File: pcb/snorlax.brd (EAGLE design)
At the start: 36.5 x 29.2 mm, 13 parts, among them IC1 MCP3008

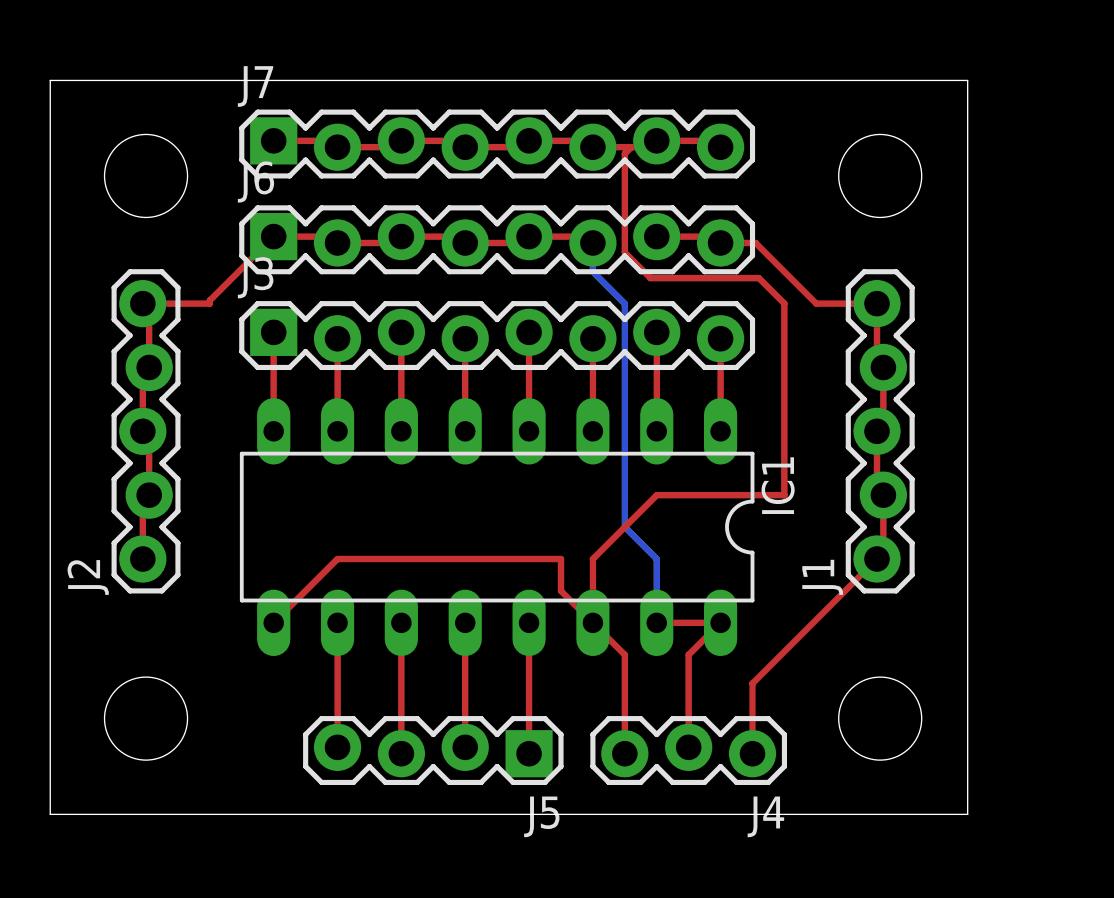
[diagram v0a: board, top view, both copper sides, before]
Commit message: Final PCB Schematics, Board Layouts and Gerber Files
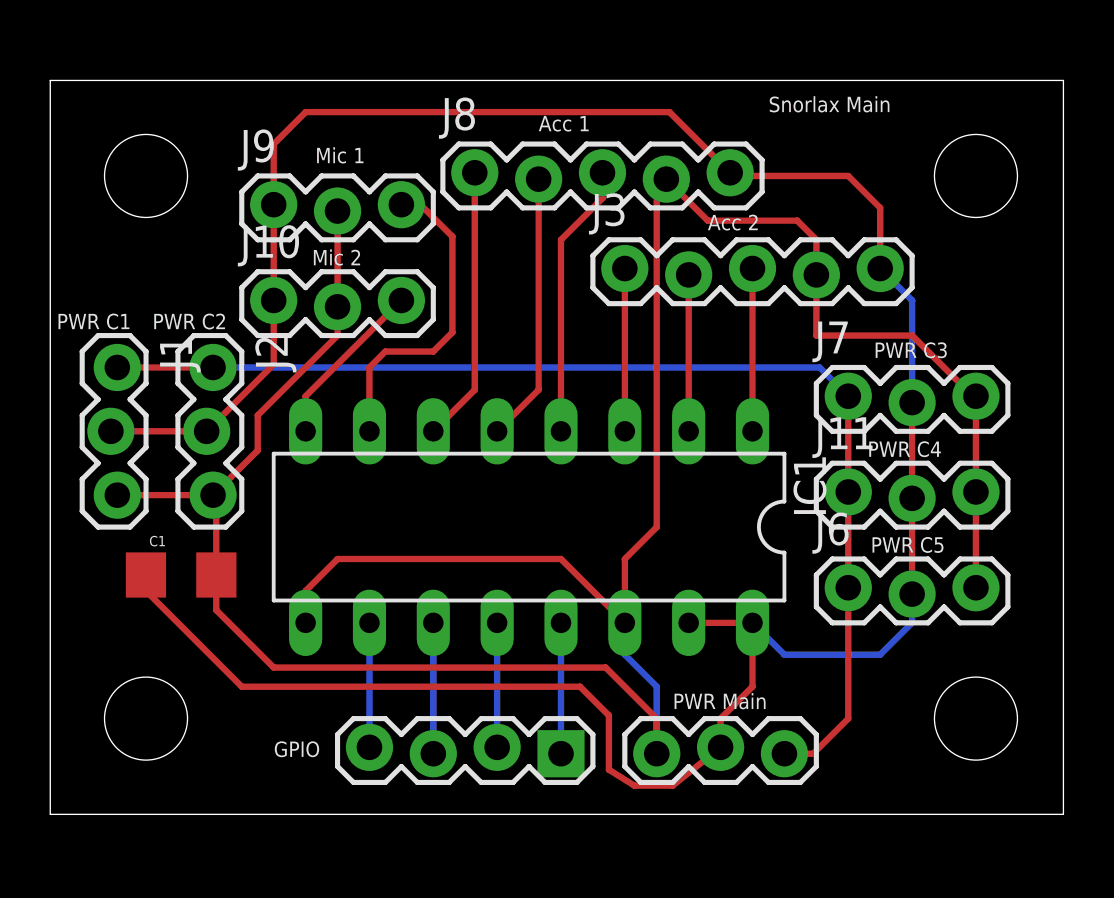
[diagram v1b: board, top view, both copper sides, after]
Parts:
- added C1: 22uF, SparkFun-Capacitors:1206
- added J10, J11, J9: (no value), SparkFun-Connectors:1X03_LOCK
- added J8: (no value), SparkFun-Connectors:1X05_LOCK
- J1, J2: device SparkFun-Connectors:1X05_LOCK -> SparkFun-Connectors:1X03_LOCK
- J3: device SparkFun-Connectors:1X08_LOCK -> SparkFun-Connectors:1X05_LOCK
- J6, J7: device SparkFun-Connectors:1X08_LOCK -> SparkFun-Connectors:1X03_LOCK
- moved J1 31.4 mm to (2.54, 17.8), turned to 270 degrees
- moved J6 26.8 mm to (31.8, 8.89)
- moved J7 25.0 mm to (31.8, 16.5)
- moved J3 14.2 mm to (22.9, 21.6)
- moved J2 8.03 mm to (6.35, 17.8), turned to 270 degrees
- moved H3 3.81 mm to (36.8, 25.4)
- moved H4 3.81 mm to (36.8, 3.81)
- moved IC1 1.27 mm to (19.1, 11.4)
- moved J4 1.27 mm to (29.2, 2.54)
- moved J5 1.27 mm to (20.3, 2.54)
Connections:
- net GND: now also C1.2, J1.3, J10.2, J11.3, J2.3, J3.4, J6.3, J8.4, J9.2; no longer J7.1, J7.2, J7.4, J7.5, J7.6, J7.7, J7.8
- net N$1: now also J3.3; no longer J3.8
- net N$2: now also J3.2; no longer J3.7
- net N$3: now also J3.1; no longer J3.6
- net N$4: now also J8.3; no longer J3.5
- net N$5: now also J8.2; no longer J3.4
- net N$6: now also J8.1; no longer J3.3
- net N$7: now also J9.3; no longer J3.2
- net N$8: now also J10.3; no longer J3.1
- net VCC_3.3: now also C1.1, J1.2, J10.1, J11.2, J3.5, J7.2, J8.5, J9.1; no longer J2.1, J2.3, J2.4, J2.5, J6.1, J6.3, J6.4, J6.5, J6.6
- net VCC_5.5: now also J11.1, J2.1, J6.1, J7.1; no longer J1.2, J1.3, J1.4, J1.5, J6.7, J6.8
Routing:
- net VCC_3.3: track 54.4 -> 103.5 mm
- net GND: track 70.1 -> 108.0 mm
- net VCC_5.5: track 30.2 -> 45.5 mm
- net N$7: track 3.68 -> 12.8 mm
- net N$5: track 3.68 -> 10.7 mm
- net N$6: track 3.94 -> 11.0 mm
- net N$4: track 3.94 -> 11.0 mm
- net N$8: track 3.94 -> 6.79 mm
- net N$3: track 3.68 -> 6.48 mm
- net N$1: track 3.68 -> 6.48 mm
- net N$2: track 3.94 -> 6.22 mm
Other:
- board size 36.5 x 29.2 mm -> 40.3 x 29.2 mm
- board text added: "Acc 1"
- board text added: "Acc 2"
- board text added: "GPIO"
- board text added: "Mic 1"
- board text added: "Mic 2"
- board text added: "PWR C1"
- board text added: "PWR C2"
- board text added: "PWR C3"
- board text added: "PWR C4"
- board text added: "PWR C5"
- board text added: "PWR Main"
- board text added: "Snorlax Main"
